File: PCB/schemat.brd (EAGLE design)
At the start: 105 x 83 mm, 58 parts, among them IC1 TEXAS_INSTRUMENTS_TLV3502AIDT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, IC2 74AC244DW, IC3 74AHC1G86DBV, IC4 7805DT

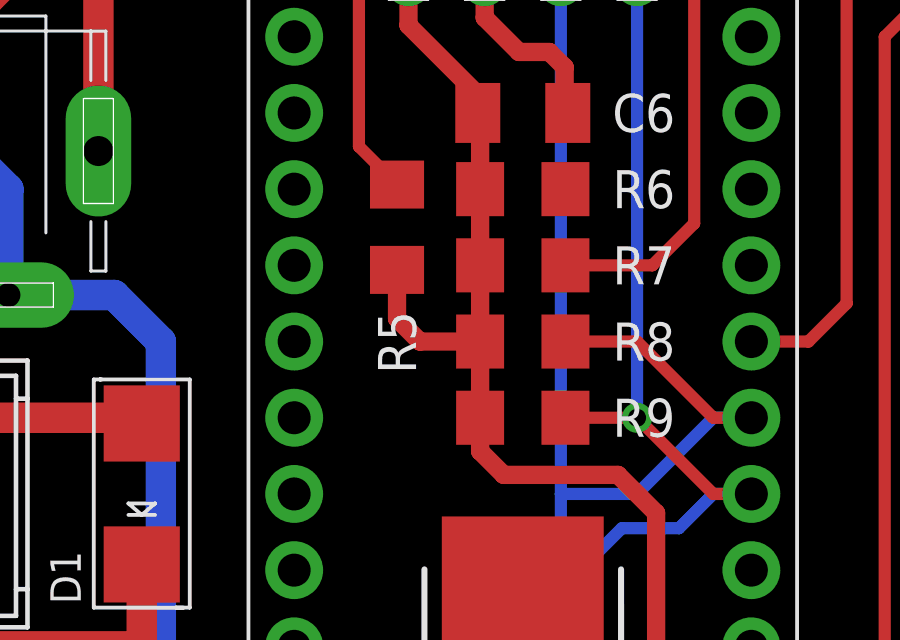
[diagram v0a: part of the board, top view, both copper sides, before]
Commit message: Praca nad rozdziałem 3
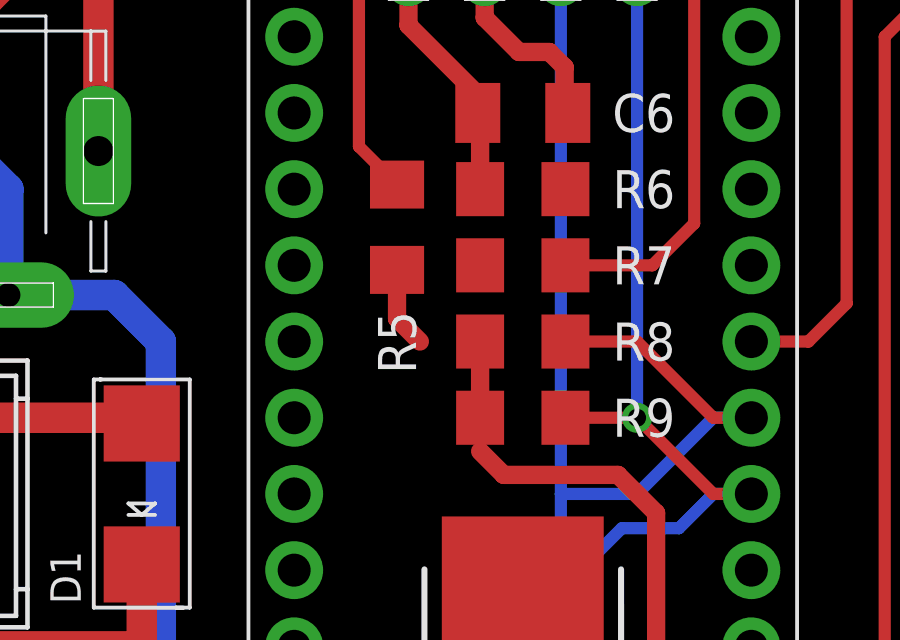
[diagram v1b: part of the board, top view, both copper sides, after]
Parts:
- D1: value (none) -> S1A
- FINGERPAD: value FINGERPAD-2B -> (none)
- FUSE: value (none) -> 750 mA
- R6: value 10k -> 5k1
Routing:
- net +5V: track 231.9 -> 223.7 mm
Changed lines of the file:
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@@
 <?xml version="1.0" encoding="utf-8"?>
 <!DOCTYPE eagle SYSTEM "eagle.dtd">
-<eagle version="9.1.2">
+<eagle version="8.0.1">
 <drawing>
 <settings>
 <setting alwaysvectorfont="no"/>
-<setting keepoldvectorfont="yes"/>
 <setting verticaltext="up"/>
 </settings>
@@
 <param name="dpMaxLengthDifference" value="10mm"/>
 <param name="dpGapFactor" value="2.5"/>
+<param name="checkGrid" value="0"/>
 <param name="checkAngle" value="0"/>
 <param name="checkFont" value="1"/>
 <param name="checkRestrict" value="1"/>
-<param name="checkStop" value="0"/>
-<param name="checkValues" value="0"/>
-<param name="checkNames" value="1"/>
-<param name="checkWireStubs" value="1"/>
-<param name="checkPolygonWidth" value="0"/>
 <param name="useDiameter" value="13"/>
 <param name="maxErrors" value="50"/>
@@
 <attribute name="VALUE" x="48.895" y="57.15" size="1.27" layer="27"/>
 </element>
-<element name="D1" library="adafruit" package="SMADIODE" value="" x="17.145" y="53.34" smashed="yes" rot="R90">
+<element name="D1" library="adafruit" package="SMADIODE" value="S1A" x="17.145" y="53.34" smashed="yes" rot="R90">
 <attribute name="NAME" x="14.097" y="51.435" size="1.016" layer="25" font="vector" rot="R270"/>
 <attribute name="VALUE" x="19.431" y="50.8" size="0.4064" layer="27" font="vector" rot="R90"/>
 </element>
-<element name="FUSE" library="adafruit" package="1812" value="" x="17.145" y="74.168" rot="R90"/>
+<element name="FUSE" library="adafruit" package="1812" value="750 mA" x="17.145" y="74.168" rot="R90"/>
 <element name="GND" library="pinhead" package="1X02" value="" x="96.25" y="24.5618" smashed="yes" rot="R270">
 <attribute name="NAME" x="99.7933" y="24.5618" size="1.27" layer="25" ratio="10" rot="R270" align="center"/>
@@
 <attribute name="VALUE" x="6.274" y="31.809" size="1.016" layer="27"/>
 </element>
-<element name="FINGERPAD" library="dom-key" package="FINGERPAD-2B" value="FINGERPAD-2B" x="9.271" y="19.812" smashed="yes" rot="R90">
+<element name="FINGERPAD" library="dom-key" package="FINGERPAD-2B" value="" x="9.271" y="19.812" smashed="yes" rot="R90">
 <attribute name="NAME" x="11.531640625" y="13.268828125" size="1.27" layer="25" font="vector" ratio="6" rot="R180"/>
 </element>
@@
 <attribute name="VALUE" x="36.83" y="66.675" size="1.27" layer="27" rot="R90"/>
 </element>
-<element name="R6" library="resistor" package="R1206" value="10k" x="29.845" y="63.5" smashed="yes" rot="R180">
+<element name="R6" library="resistor" package="R1206" value="5k1" x="29.845" y="63.5" smashed="yes" rot="R180">
 <attribute name="NAME" x="34.925" y="64.135" size="1.27" layer="25" rot="R180"/>
 <attribute name="VALUE" x="31.115" y="66.04" size="1.27" layer="27" rot="R180"/>
@@
 <contactref element="IC2" pad="20"/>
 <contactref element="C7" pad="1"/>
-<contactref element="R9" pad="2"/>
-<contactref element="R8" pad="2"/>
-<contactref element="R7" pad="2"/>
 <contactref element="R1" pad="2"/>
 <contactref element="R3" pad="2"/>
@@
 <wire x1="33.3" y1="42.19" x2="32.125" y2="42.19" width="0.6096" layer="1"/>
 <wire x1="34.29" y1="43.18" x2="33.3" y2="42.19" width="0.6096" layer="1"/>
-<wire x1="28.423" y1="58.42" x2="28.423" y2="60.96" width="0.6096" layer="1"/>
-<wire x1="28.423" y1="58.42" x2="28.423" y2="55.88" width="0.6096" layer="1"/>
 <wire x1="32.125" y1="42.19" x2="32.125" y2="40.395" width="1.016" layer="1"/>
 <wire x1="32.125" y1="40.395" x2="33.02" y2="39.6" width="1.016" layer="1"/>
@@
 <wire x1="14.605" y1="36.195" x2="17.145" y2="33.655" width="1.016" layer="1"/>
 <contactref element="C6" pad="1"/>
-<wire x1="28.423" y1="60.96" x2="28.423" y2="63.5" width="0.6096" layer="1"/>
 <wire x1="28.423" y1="63.5" x2="28.423" y2="66.018" width="0.6096" layer="1"/>
 <wire x1="28.423" y1="66.018" x2="28.345" y2="66.04" width="0.6096" layer="1"/>
@@
 <wire x1="25.654" y1="60.808" x2="25.654" y2="59.182" width="0.6096" layer="1"/>
 <wire x1="25.654" y1="59.182" x2="26.416" y2="58.42" width="0.6096" layer="1"/>
-<wire x1="26.416" y1="58.42" x2="28.423" y2="58.42" width="0.6096" layer="1"/>
 <wire x1="63.497" y1="50.8" x2="63.5" y2="50.803" width="1.016" layer="1"/>
 <wire x1="63.5" y1="50.803" x2="69.215" y2="50.803" width="1.016" layer="1"/>
@@
 <wire x1="29.21" y1="78.74" x2="37.465" y2="78.74" width="0.6096" layer="1"/>
 <wire x1="26.035" y1="75.565" x2="29.21" y2="78.74" width="0.6096" layer="1"/>
-<wire x1="28.423" y1="55.88" x2="28.423" y2="54.762" width="0.6096" layer="1"/>
 <wire x1="28.423" y1="54.762" x2="29.21" y2="53.975" width="0.6096" layer="1"/>
 <wire x1="29.21" y1="53.975" x2="33.02" y2="53.975" width="0.6096" layer="1"/>
@@
 <wire x1="14.605" y1="36.195" x2="8.001" y2="36.195" width="1.016" layer="1"/>
 <wire x1="8.001" y1="36.195" x2="6.35" y2="34.544" width="1.016" layer="1"/>
+<contactref element="R9" pad="2"/>
+<contactref element="R8" pad="2"/>
+<contactref element="R7" pad="2"/>
+<wire x1="28.423" y1="58.42" x2="28.423" y2="55.88" width="0.6096" layer="1"/>
+<wire x1="28.423" y1="60.96" x2="28.423" y2="63.5" width="0" layer="19" extent="1-1"/>
+<wire x1="28.423" y1="58.42" x2="28.423" y2="60.96" width="0" layer="19" extent="1-1"/>
+<wire x1="28.423" y1="54.762" x2="28.423" y2="55.88" width="0" layer="19" extent="1-1"/>
+<wire x1="26.416" y1="58.42" x2="28.423" y2="58.42" width="0" layer="19" extent="1-1"/>
 </signal>
 <signal name="GND">
@@
 </signal>
 </signals>
-<mfgpreviewcolors>
-<mfgpreviewcolor name="soldermaskcolor" color="0xC8008000"/>
-<mfgpreviewcolor name="silkscreencolor" color="0xFFFEFEFE"/>
-<mfgpreviewcolor name="backgroundcolor" color="0xFF282828"/>
-<mfgpreviewcolor name="coppercolor" color="0xFFFFBF00"/>
-<mfgpreviewcolor name="substratecolor" color="0xFF786E46"/>
-</mfgpreviewcolors>
 <errors>
 </errors>
